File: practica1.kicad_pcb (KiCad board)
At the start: 2 copper layers, 0 parts

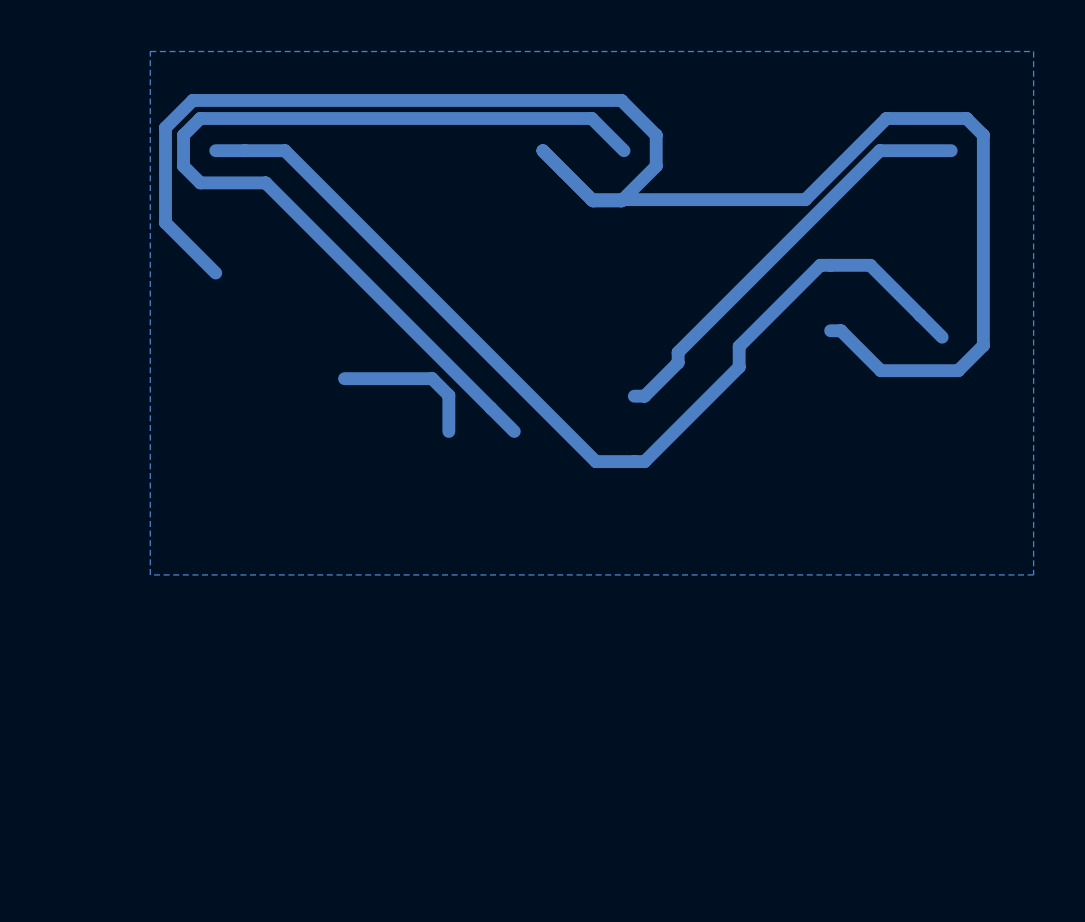
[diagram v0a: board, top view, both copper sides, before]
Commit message: 3D
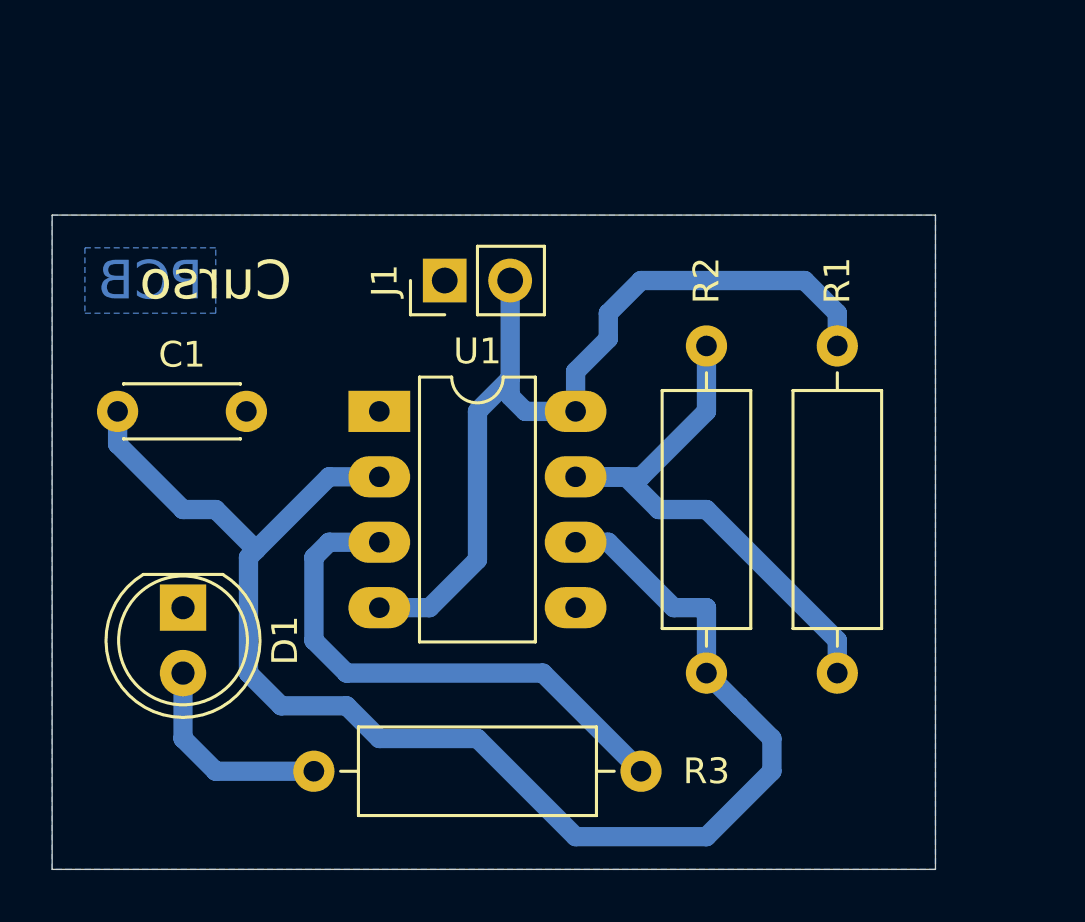
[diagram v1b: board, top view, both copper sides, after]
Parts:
- added C1: 0.15uF, Capacitor_THT:C_Disc_D4.3mm_W1.9mm_P5.00mm, F.Cu at (133.3, 114.3)
- added D1: LED RED, LED_THT:LED_D5.0mm, F.Cu at (135.9, 121.9)
- added J1: 5V, Connector_PinHeader_2.54mm:PinHeader_1x02_P2.54mm_Vertical, F.Cu at (146.1, 109.2)
- added R1: 5k, Resistor_THT:R_Axial_DIN0309_L9.0mm_D3.2mm_P12.70mm_Horizontal, F.Cu at (161.3, 111.8)
- added R2: 3k, Resistor_THT:R_Axial_DIN0309_L9.0mm_D3.2mm_P12.70mm_Horizontal, F.Cu at (156.2, 111.8)
- added R3: 330, Resistor_THT:R_Axial_DIN0309_L9.0mm_D3.2mm_P12.70mm_Horizontal, F.Cu at (141.0, 128.3)
- added U1: NE555, Package_DIP:DIP-8_W7.62mm_LongPads, F.Cu at (143.5, 114.3)
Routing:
- net Net-(C1-Pad1): track 0.00 -> 56.7 mm
- net Net-(R1-Pad2): track 68.1 -> 22.7 mm
- net Net-(D1-Pad2): track 36.2 -> 8.15 mm
- net GND: track 5.72 -> 0.00 mm
- net /Salida: track 16.5 -> 20.8 mm
- net +5V: track 38.0 -> 35.0 mm
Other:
- board outline added: 34.3 x 25.4 mm
- board text added: "Curso"
- board text added: "PCB"
- board text added: "V1.0"
